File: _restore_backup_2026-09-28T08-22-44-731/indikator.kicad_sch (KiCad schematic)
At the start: 104 parts, among them J1 Conn_01x02, Q1 AO3400A, Q10 AO3400A, Q11 AO3400A, Q12 AO3400A, Q13 AO3400A, Q14 AO3400A, Q15 AO3400A, Q16 AO3400A, Q17 AO3400A, Q18 AO3400A, Q19 AO3400A, Q2 AO3400A, Q20 AO3400A, Q21 AO3400A, Q22 AO3400A, Q23 AO3400A, Q24 AO3400A, Q3 AO3400A, Q4 AO3400A, Q5 AO3400A, Q6 AO3400A, Q7 AO3400A, Q8 AO3400A, Q9 AO3400A, U1 XIAO-ESP32-C3-SMD, U2 74HC595, U3 74HC595, U4 74HC595

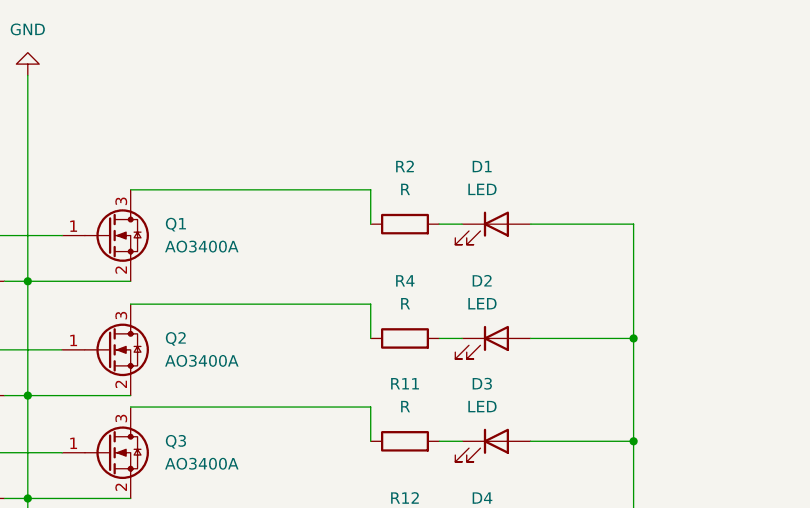
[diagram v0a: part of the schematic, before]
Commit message: ROUTING IS FRICKIN IMPOSSIBLE BRUH
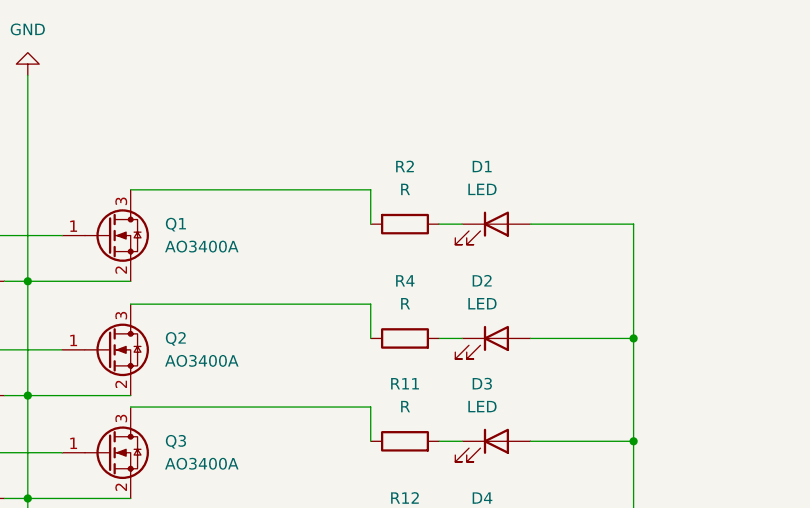
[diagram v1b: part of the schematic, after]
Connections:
- net at D1.1 (K): now also R2.1; no longer R2.2
- net at Q1.3 (D): now also R2.2; no longer R2.1
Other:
- moved on the sheet: R2
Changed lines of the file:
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@@
 	(symbol
 		(lib_id "Device:R")
-		(at 237.49 59.69 90)
+		(at 237.49 59.69 270)
 		(unit 1)
 		(body_style 1)
@@
 		)
 		(property "Footprint" "Resistor_SMD:R_0805_2012Metric"
-			(at 237.49 61.468 90)
+			(at 237.49 57.912 90)
 			(hide yes)
 			(show_name no)
